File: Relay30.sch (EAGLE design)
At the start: 33 parts

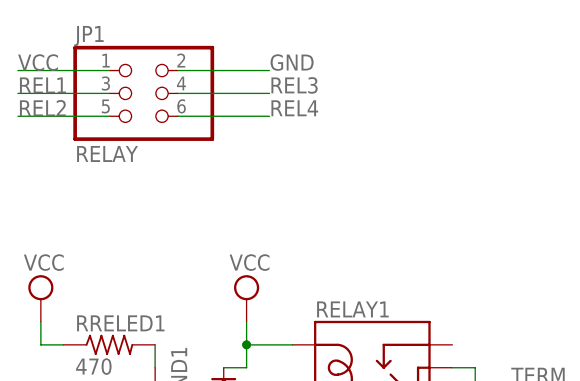
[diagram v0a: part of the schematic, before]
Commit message: 11/10/3
FIXED:
-connector
-refine route
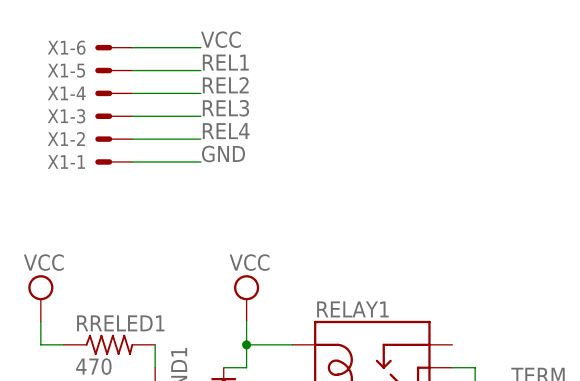
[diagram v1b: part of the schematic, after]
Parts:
- removed JP1: RELAY, pinhead:PINHD-2X3
- added X1: (no value), con-molex:22-23-2061
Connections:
- net GND: now also X1-1.S; no longer JP1.2
- net REL1: now also X1-5.S; no longer JP1.3
- net REL2: now also X1-4.S; no longer JP1.5
- net REL3: now also X1-3.S; no longer JP1.4
- net REL4: now also X1-2.S; no longer JP1.6
- net VCC: now also X1-6.S; no longer JP1.1
